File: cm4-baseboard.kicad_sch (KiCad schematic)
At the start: 4 parts

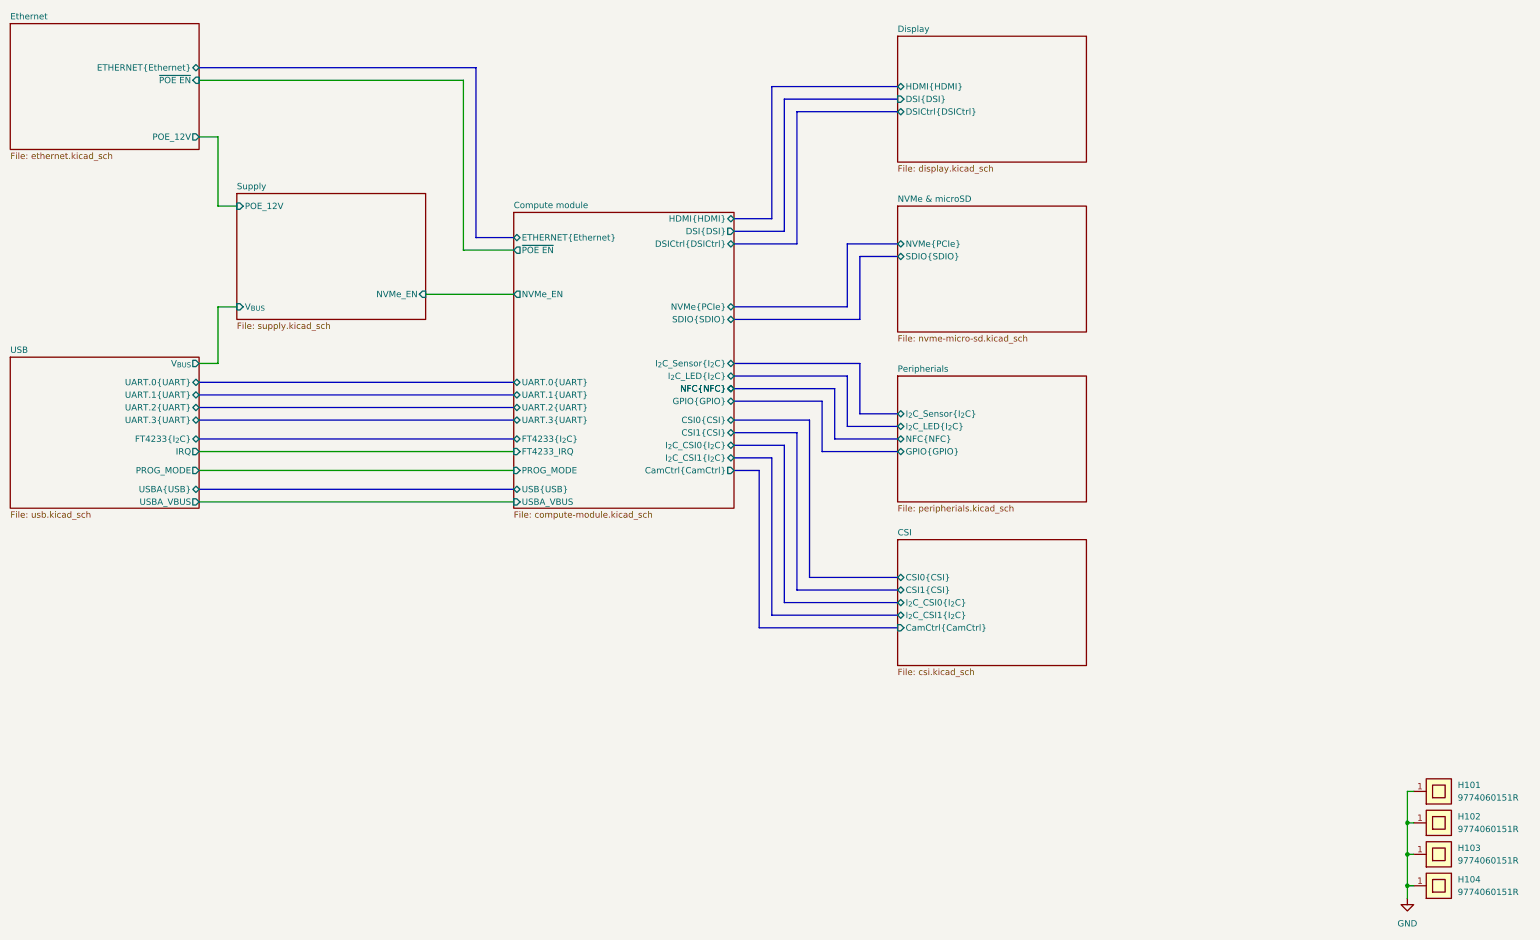
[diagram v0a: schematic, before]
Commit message: [#55532] Sch: Optimize conections for easier routing
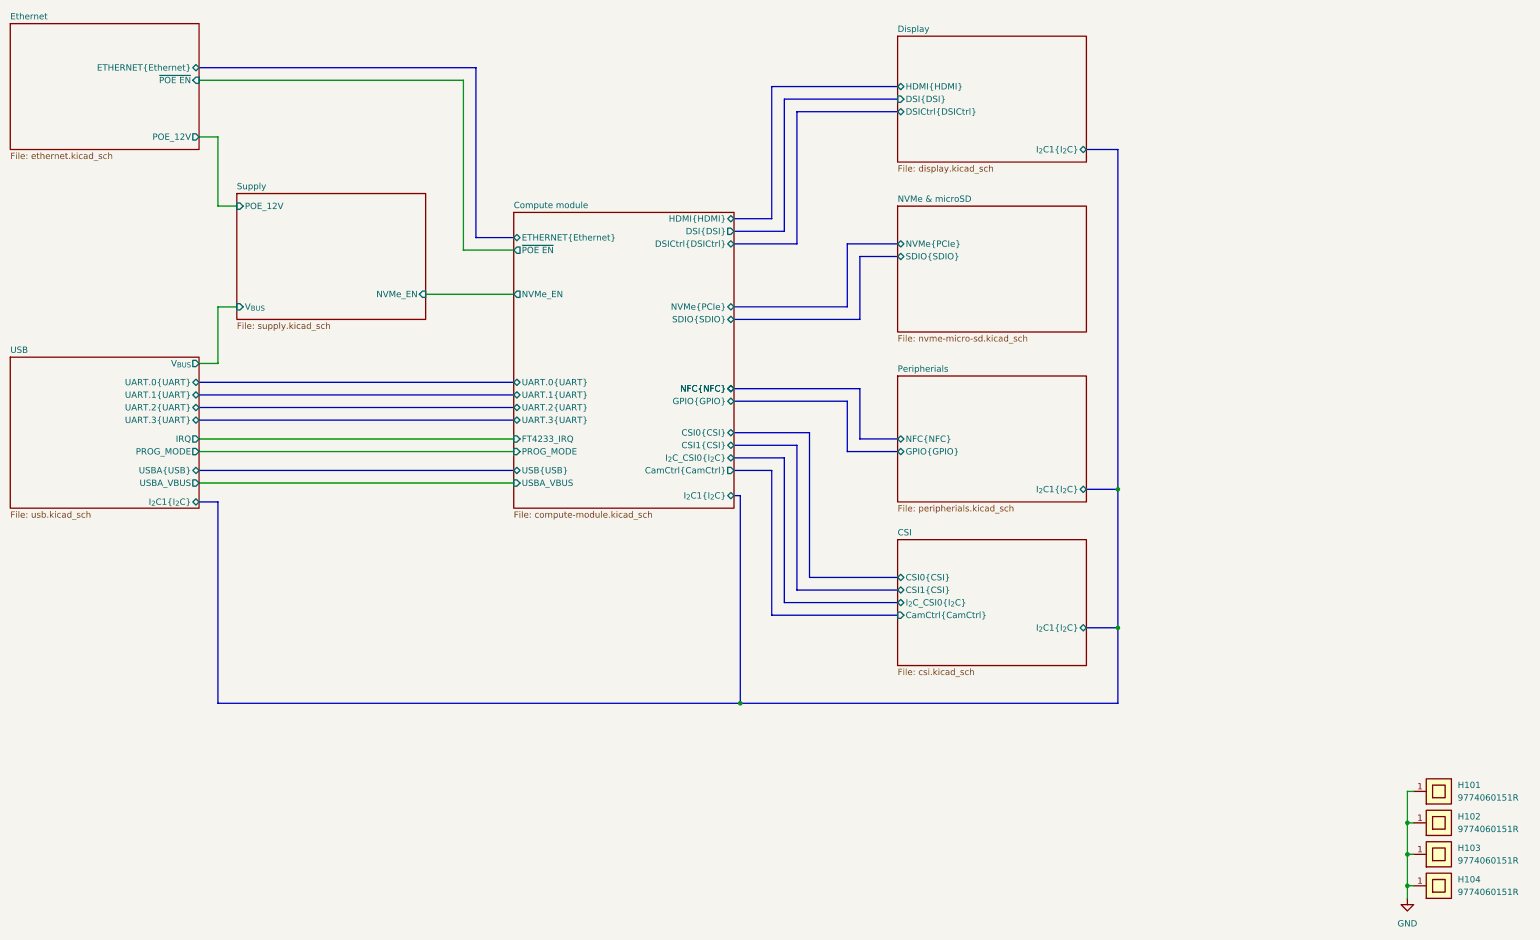
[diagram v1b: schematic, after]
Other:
- sheet CSI ports: added I_{2}C1{I_{2}C}; removed I_{2}C_CSI1{I_{2}C}
- sheet Compute module ports: added I_{2}C1{I_{2}C}; removed FT4233{I_{2}C}, I_{2}C_CSI1{I_{2}C}, I_{2}C_LED{I_{2}C}, I_{2}C_Sensor{I_{2}C}
- sheet Display ports: added I_{2}C1{I_{2}C}; removed none
- sheet Peripherials ports: added I_{2}C1{I_{2}C}; removed I_{2}C_LED{I_{2}C}, I_{2}C_Sensor{I_{2}C}
- sheet USB ports: added I_{2}C1{I_{2}C}; removed FT4233{I_{2}C}
